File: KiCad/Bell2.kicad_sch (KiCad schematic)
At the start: 34 parts, among them J1 USB-C, J2 POWER, J3 Conn_01x10, U1 ESP32-PICO-MINI-02, U2 FT231XQ, U3 ISL89410, U4 ISL89410, U5 LMR16006+FB, U6 AA, U7 QR

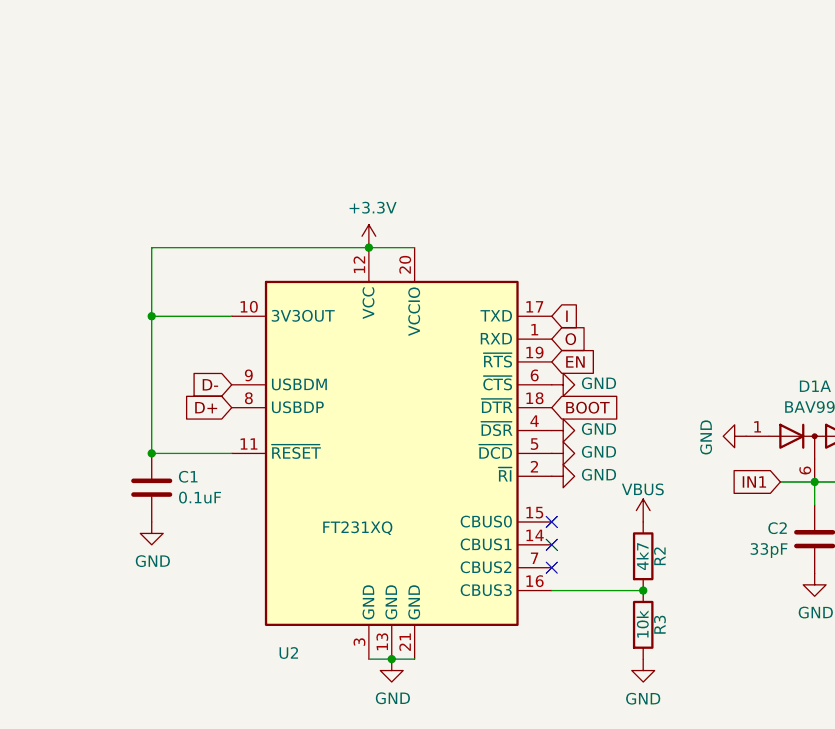
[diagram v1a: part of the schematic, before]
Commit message: Tidy
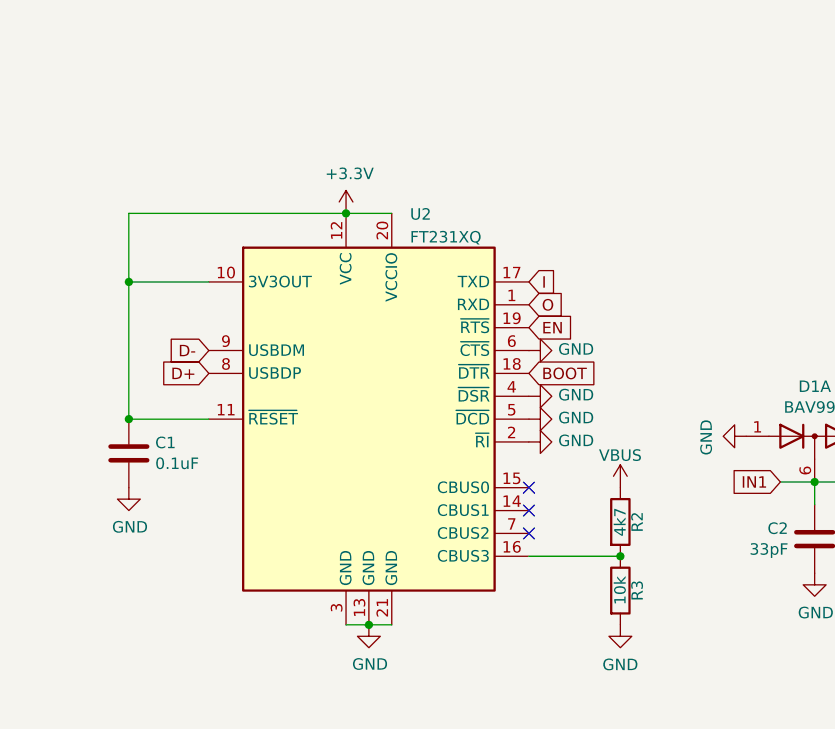
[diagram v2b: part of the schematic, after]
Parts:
- removed U2: FT231XQ, Package_DFN_QFN:QFN-20-1EP_4x4mm_P0.5mm_EP2.5x2.5mm, symbol Interface_USB:FT231XQ
- added U2: FT231XQ, RevK:QFN-20-1EP_4x4mm_P0.5mm_EP2.5x2.5mm, symbol RevK:FT231XQ
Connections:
- net +3V3: now also U2.10 (3V3OUT), U2.11 (~{RESET}), U2.12 (VCC), U2.20 (VCCIO)
- net BOOT: now also U2.18 (~{DTR})
- net D+: now also U2.8 (USBDP)
- net D-: now also U2.9 (USBDM)
- net EN: now also U2.19 (~{RTS})
- net GND: now also U2.13 (GND), U2.2 (~{RI}), U2.21 (GND), U2.3 (GND), U2.4 (~{DSR}), U2.5 (~{DCD}), U2.6 (~{CTS})
- net I: now also U2.17 (TXD)
- net O: now also U2.1 (RXD)
- net at R2.2, R3.1: now also U2.16 (CBUS3)
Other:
- moved on the sheet: C1, R2, R3
